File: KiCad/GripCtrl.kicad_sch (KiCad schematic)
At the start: 18 parts, among them SW1 SW_Push, SW10 SW_Push, SW11 SW_Push, SW2 SW_Push, SW3 SW_Push, SW4 SW_Push, SW5 SW_Push, SW6 SW_Push, SW7 SW_Push, SW8 SW_Push, SW9 SW_Push, U1 ESP32-DevKitC, U2 NRF24L01_

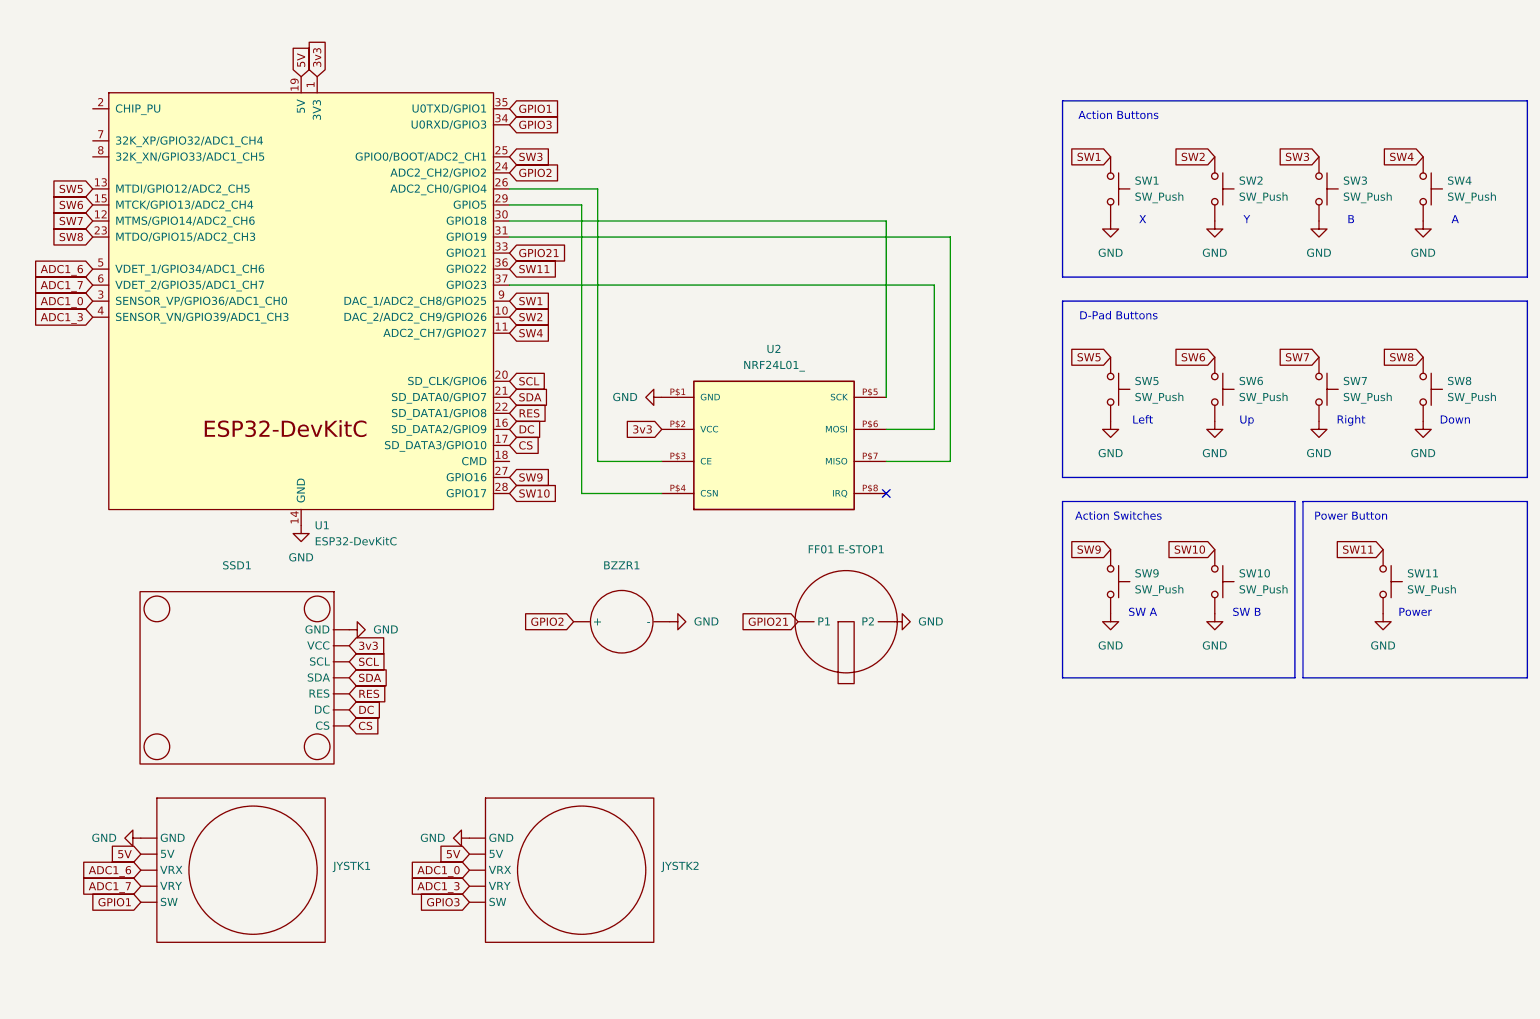
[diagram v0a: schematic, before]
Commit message: Update schematic
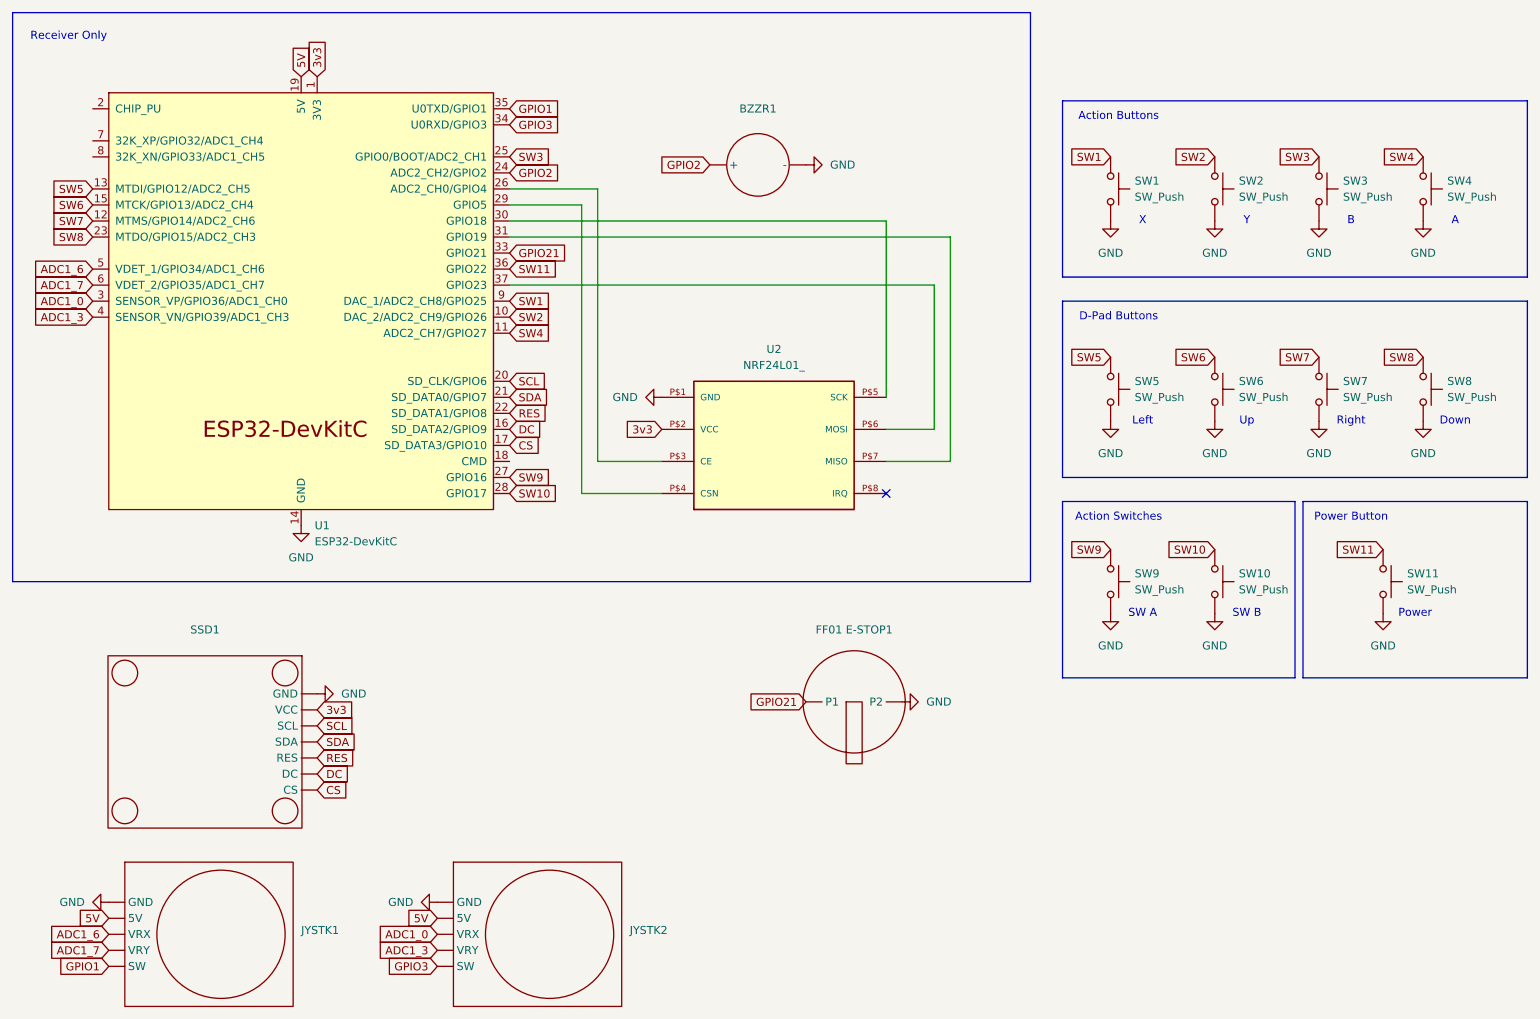
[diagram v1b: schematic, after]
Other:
- note added: "Receiver Only"
- moved on the sheet: BZZR1, FF01 E-STOP1, JYSTK1, JYSTK2, SSD1
